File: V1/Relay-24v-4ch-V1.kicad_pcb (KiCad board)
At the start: 2 copper layers, 53 x 67.8 mm, 25 parts, among them J1 Conn_01x05, J2 OUT1, J3 OUT2, J4 OUT3, J5 OUT4, K1 G5PZ-1A, K2 G5PZ-1A, K3 G5PZ-1A, K4 G5PZ-1A

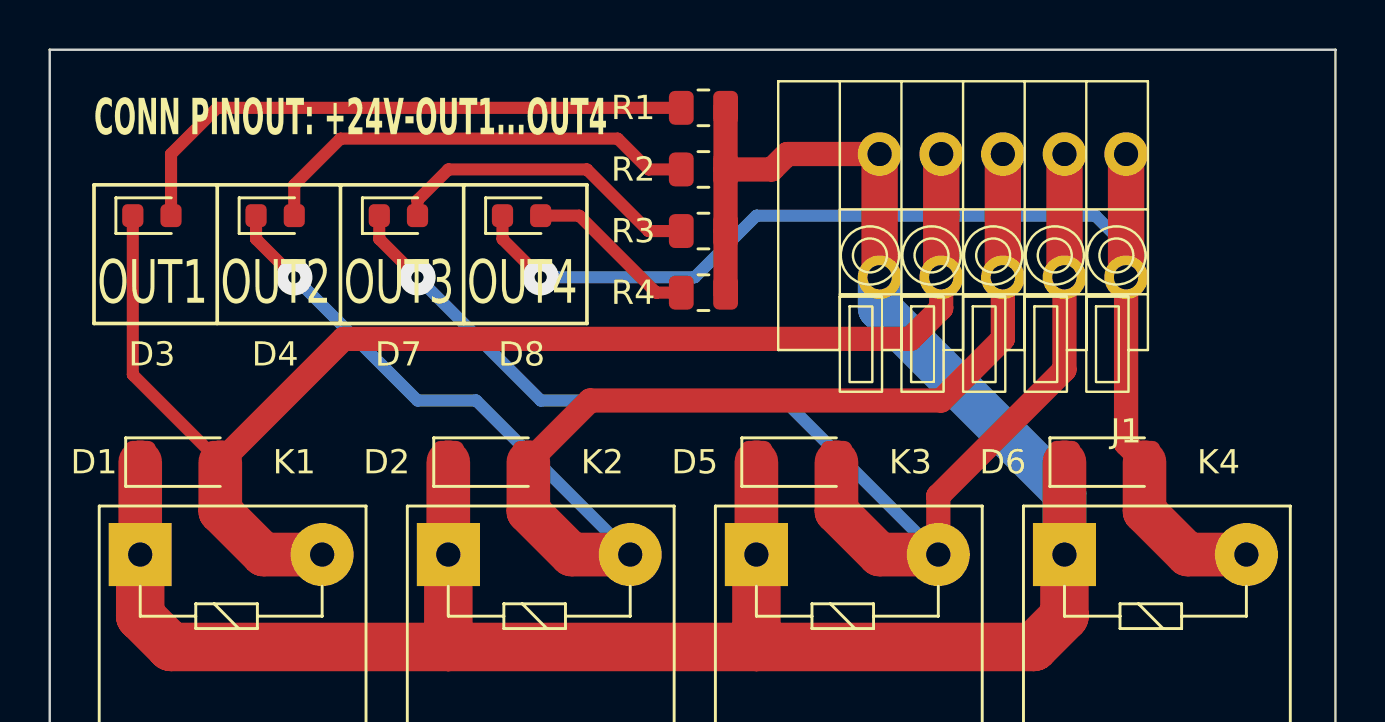
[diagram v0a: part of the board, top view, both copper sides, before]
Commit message: Update board images
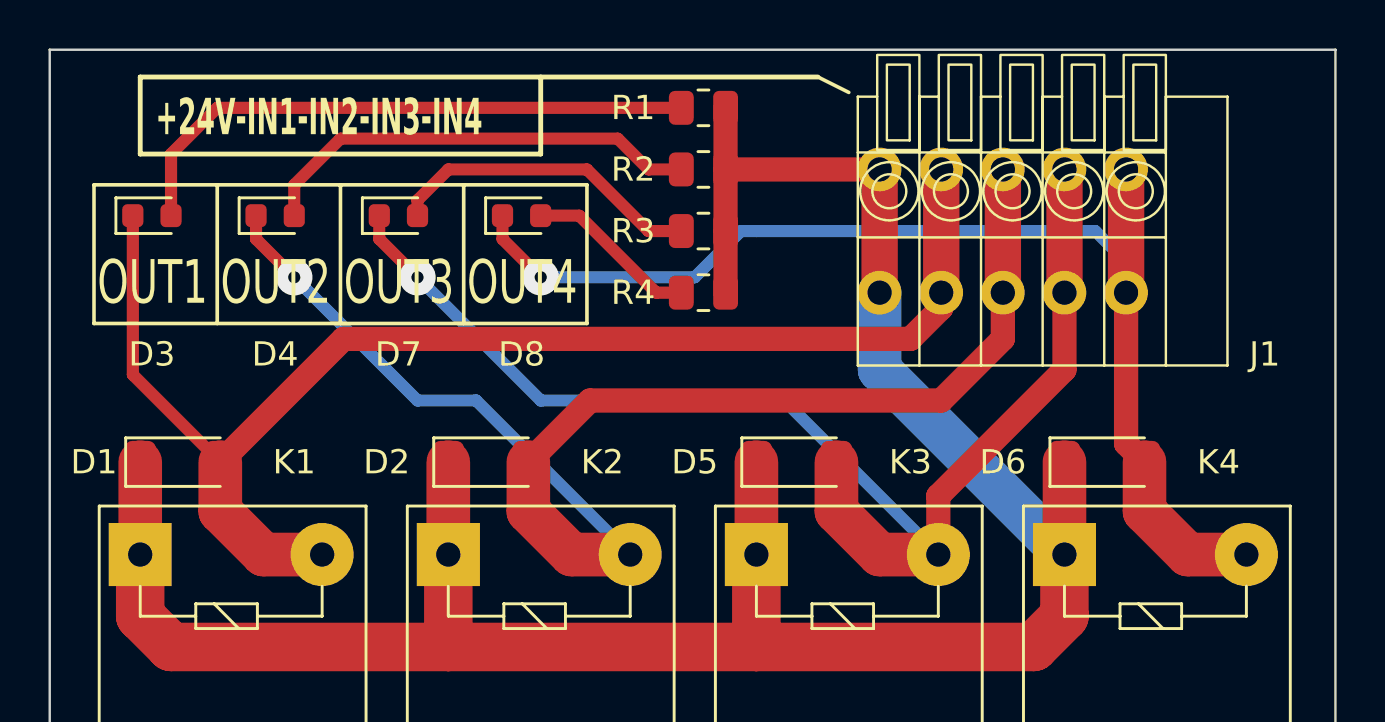
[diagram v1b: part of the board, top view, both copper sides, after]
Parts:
- moved J1 11.1 mm to (141.0, 62.9), turned to 180 degrees
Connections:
- J1 pad 1: +24V -> Net-(D6-A)
- J1 pad 2: Net-(D1-A) -> Net-(D5-A)
- J1 pad 4: Net-(D5-A) -> Net-(D1-A)
- J1 pad 5: Net-(D6-A) -> +24V
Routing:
- net +24V: track 101.0 -> 100.1 mm
- net Net-(D1-A): track 57.3 -> 56.7 mm
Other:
- board text added: "+24V-IN1-IN2-IN3-IN4"
- board text removed: "CONN PINOUT: +24V-OUT1...OUT4"
